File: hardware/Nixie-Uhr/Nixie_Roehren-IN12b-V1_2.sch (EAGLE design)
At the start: 21 parts

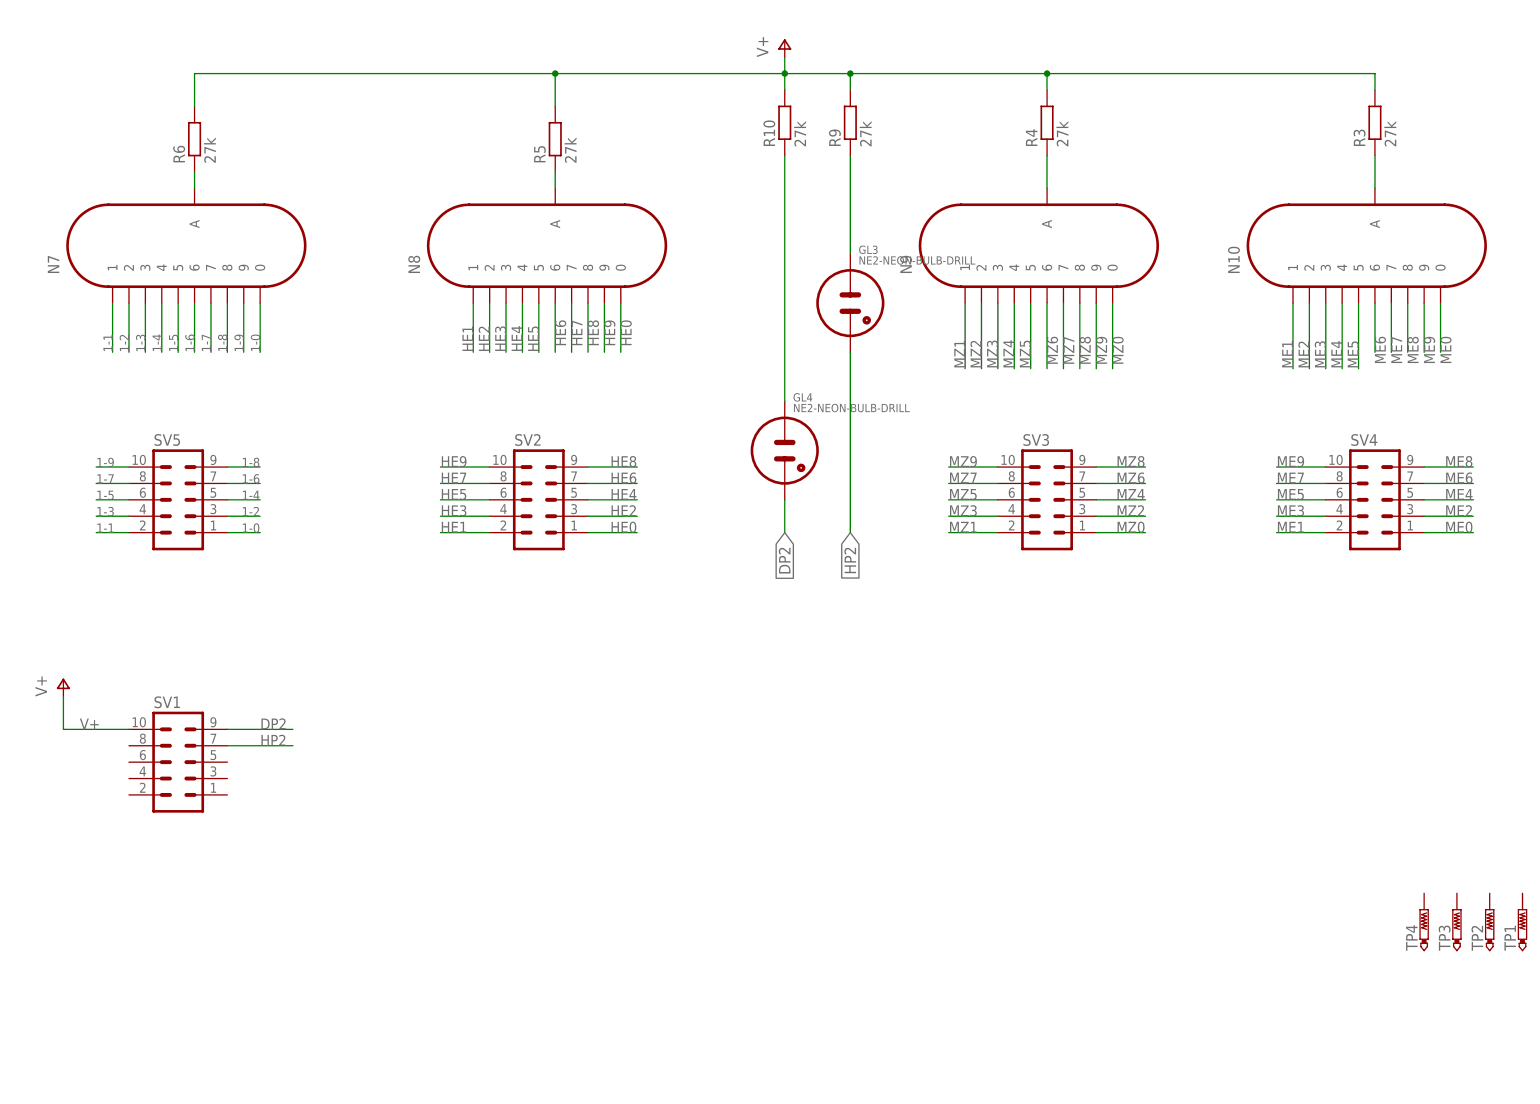
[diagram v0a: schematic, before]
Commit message: Hardware description updated.
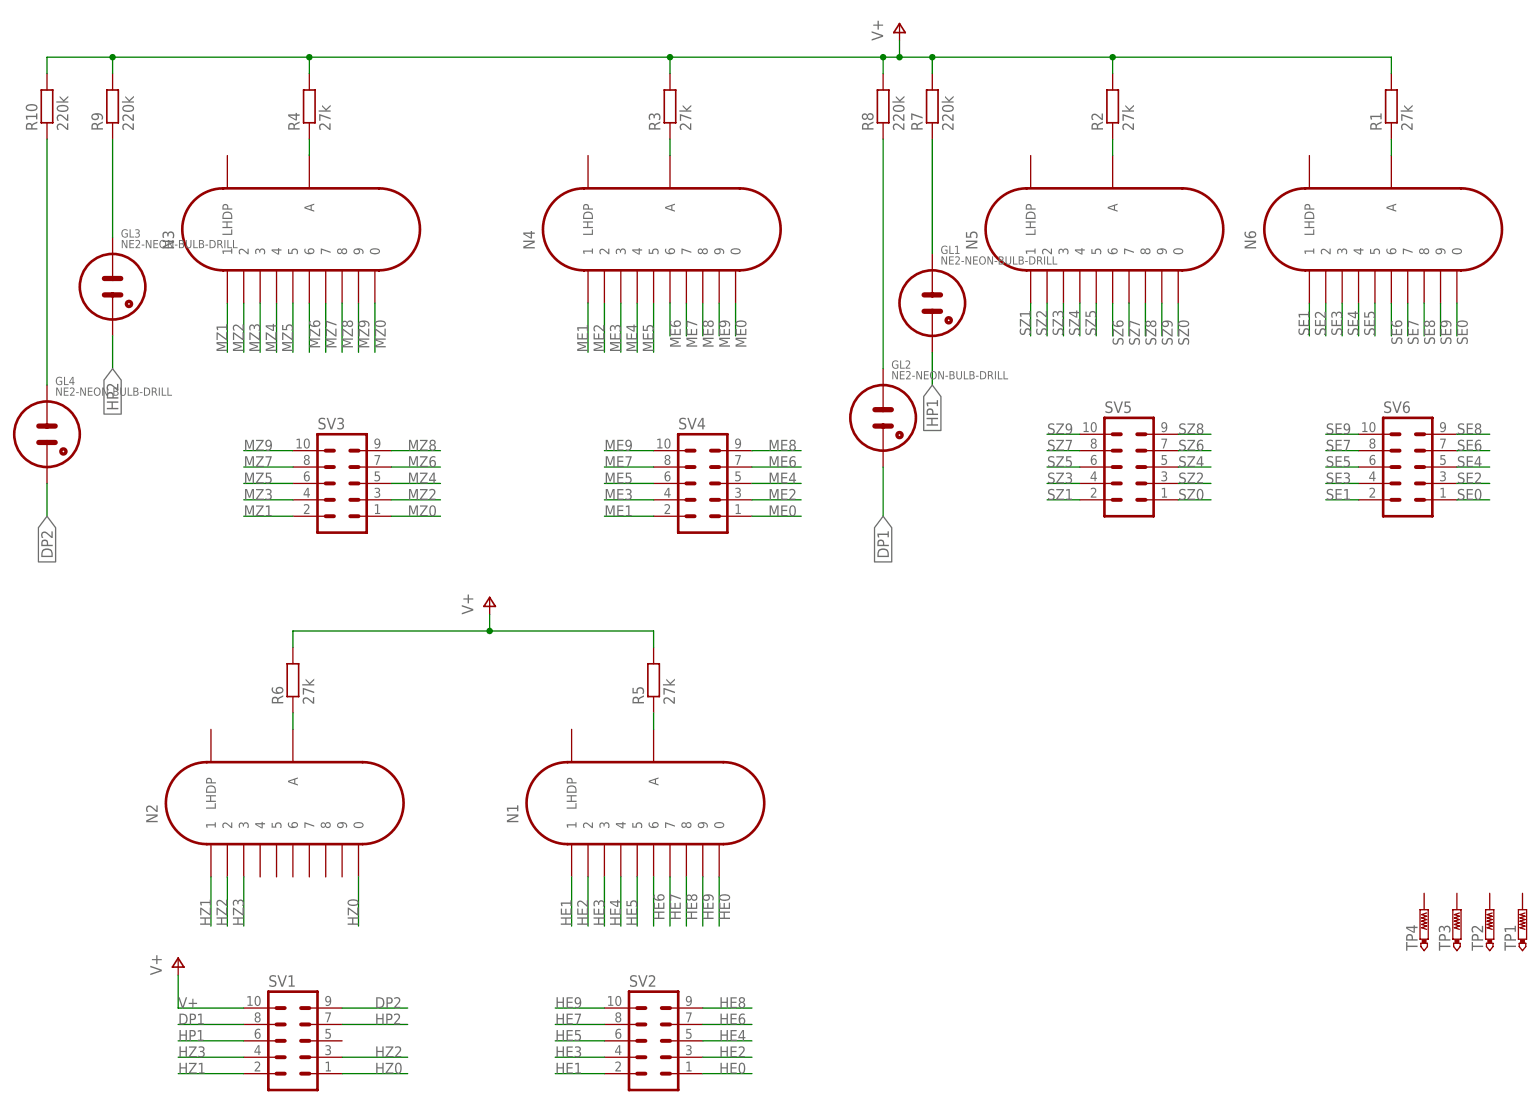
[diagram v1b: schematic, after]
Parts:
- removed N10, N7, N8, N9: IN-1A, russian-nixies:IN-1A
- added GL1, GL2: NE2-NEON-BULB-DRILL, nixies:NE2-NEON-BULB-DRILL
- added N1, N2, N3, N4, N5, N6: IN-12B, russian-nixies:IN-12B
- added R1, R2: 27k, rcl:R-EU_0207/10
- added R7, R8: 220k, rcl:R-EU_0207/10
- added SV6: (no value), con-harting-ml:ML10
- R10, R9: value 27k -> 220k
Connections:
- removed net 1-0: N7.0, SV5.1
- removed net 1-1: N7.1, SV5.2
- removed net 1-2: N7.2, SV5.3
- removed net 1-3: N7.3, SV5.4
- removed net 1-4: N7.4, SV5.5
- removed net 1-5: N7.5, SV5.6
- removed net 1-6: N7.6, SV5.7
- removed net 1-7: N7.7, SV5.8
- removed net 1-8: N7.8, SV5.9
- removed net 1-9: N7.9, SV5.10
- new net DP1: GL2.A1, SV1.8
- new net HP1: GL1.A1, SV1.6
- new net HZ0: N2.0, SV1.1
- new net HZ1: N2.1, SV1.2
- new net HZ2: N2.2, SV1.3
- new net HZ3: N2.3, SV1.4
- new net N$2: N6.A, R1.1
- new net N$3: N5.A, R2.1
- new net N$6: GL2.A, R8.1
- new net N$8: GL1.A, R7.1
- new net SE0: N6.0, SV6.1
- new net SE1: N6.1, SV6.2
- new net SE2: N6.2, SV6.3
- new net SE3: N6.3, SV6.4
- new net SE4: N6.4, SV6.5
- new net SE5: N6.5, SV6.6
- new net SE6: N6.6, SV6.7
- new net SE7: N6.7, SV6.8
- new net SE8: N6.8, SV6.9
- new net SE9: N6.9, SV6.10
- new net SZ0: N5.0, SV5.1
- new net SZ1: N5.1, SV5.2
- new net SZ2: N5.2, SV5.3
- new net SZ3: N5.3, SV5.4
- new net SZ4: N5.4, SV5.5
- new net SZ5: N5.5, SV5.6
- new net SZ6: N5.6, SV5.7
- new net SZ7: N5.7, SV5.8
- new net SZ8: N5.8, SV5.9
- new net SZ9: N5.9, SV5.10
- net HE0: now also N1.0; no longer N8.0
- net HE1: now also N1.1; no longer N8.1
- net HE2: now also N1.2; no longer N8.2
- net HE3: now also N1.3; no longer N8.3
- net HE4: now also N1.4; no longer N8.4
- net HE5: now also N1.5; no longer N8.5
- net HE6: now also N1.6; no longer N8.6
- net HE7: now also N1.7; no longer N8.7
- net HE8: now also N1.8; no longer N8.8
- net HE9: now also N1.9; no longer N8.9
- net ME0: now also N4.0; no longer N10.0
- net ME1: now also N4.1; no longer N10.1
- net ME2: now also N4.2; no longer N10.2
- net ME3: now also N4.3; no longer N10.3
- net ME4: now also N4.4; no longer N10.4
- net ME5: now also N4.5; no longer N10.5
- net ME6: now also N4.6; no longer N10.6
- net ME7: now also N4.7; no longer N10.7
- net ME8: now also N4.8; no longer N10.8
- net ME9: now also N4.9; no longer N10.9
- net MZ0: now also N3.0; no longer N9.0
- net MZ1: now also N3.1; no longer N9.1
- net MZ2: now also N3.2; no longer N9.2
- net MZ3: now also N3.3; no longer N9.3
- net MZ4: now also N3.4; no longer N9.4
- net MZ5: now also N3.5; no longer N9.5
- net MZ6: now also N3.6; no longer N9.6
- net MZ7: now also N3.7; no longer N9.7
- net MZ8: now also N3.8; no longer N9.8
- net MZ9: now also N3.9; no longer N9.9
- net N$1: now also N2.A; no longer N7.A
- net N$4: now also N4.A; no longer N10.A
- net N$5: now also N3.A; no longer N9.A
- net N$7: now also N1.A; no longer N8.A
- net V+: now also R1.2, R2.2, R7.2, R8.2
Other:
- moved on the sheet: GL3, GL4, R10, R3, R4, R5, R6, R9, SV1, SV2, SV3, SV4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
